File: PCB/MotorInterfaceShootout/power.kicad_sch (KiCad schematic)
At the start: 19 parts, among them U2 OPA4197, U3 LM7810, U4 LM79L05

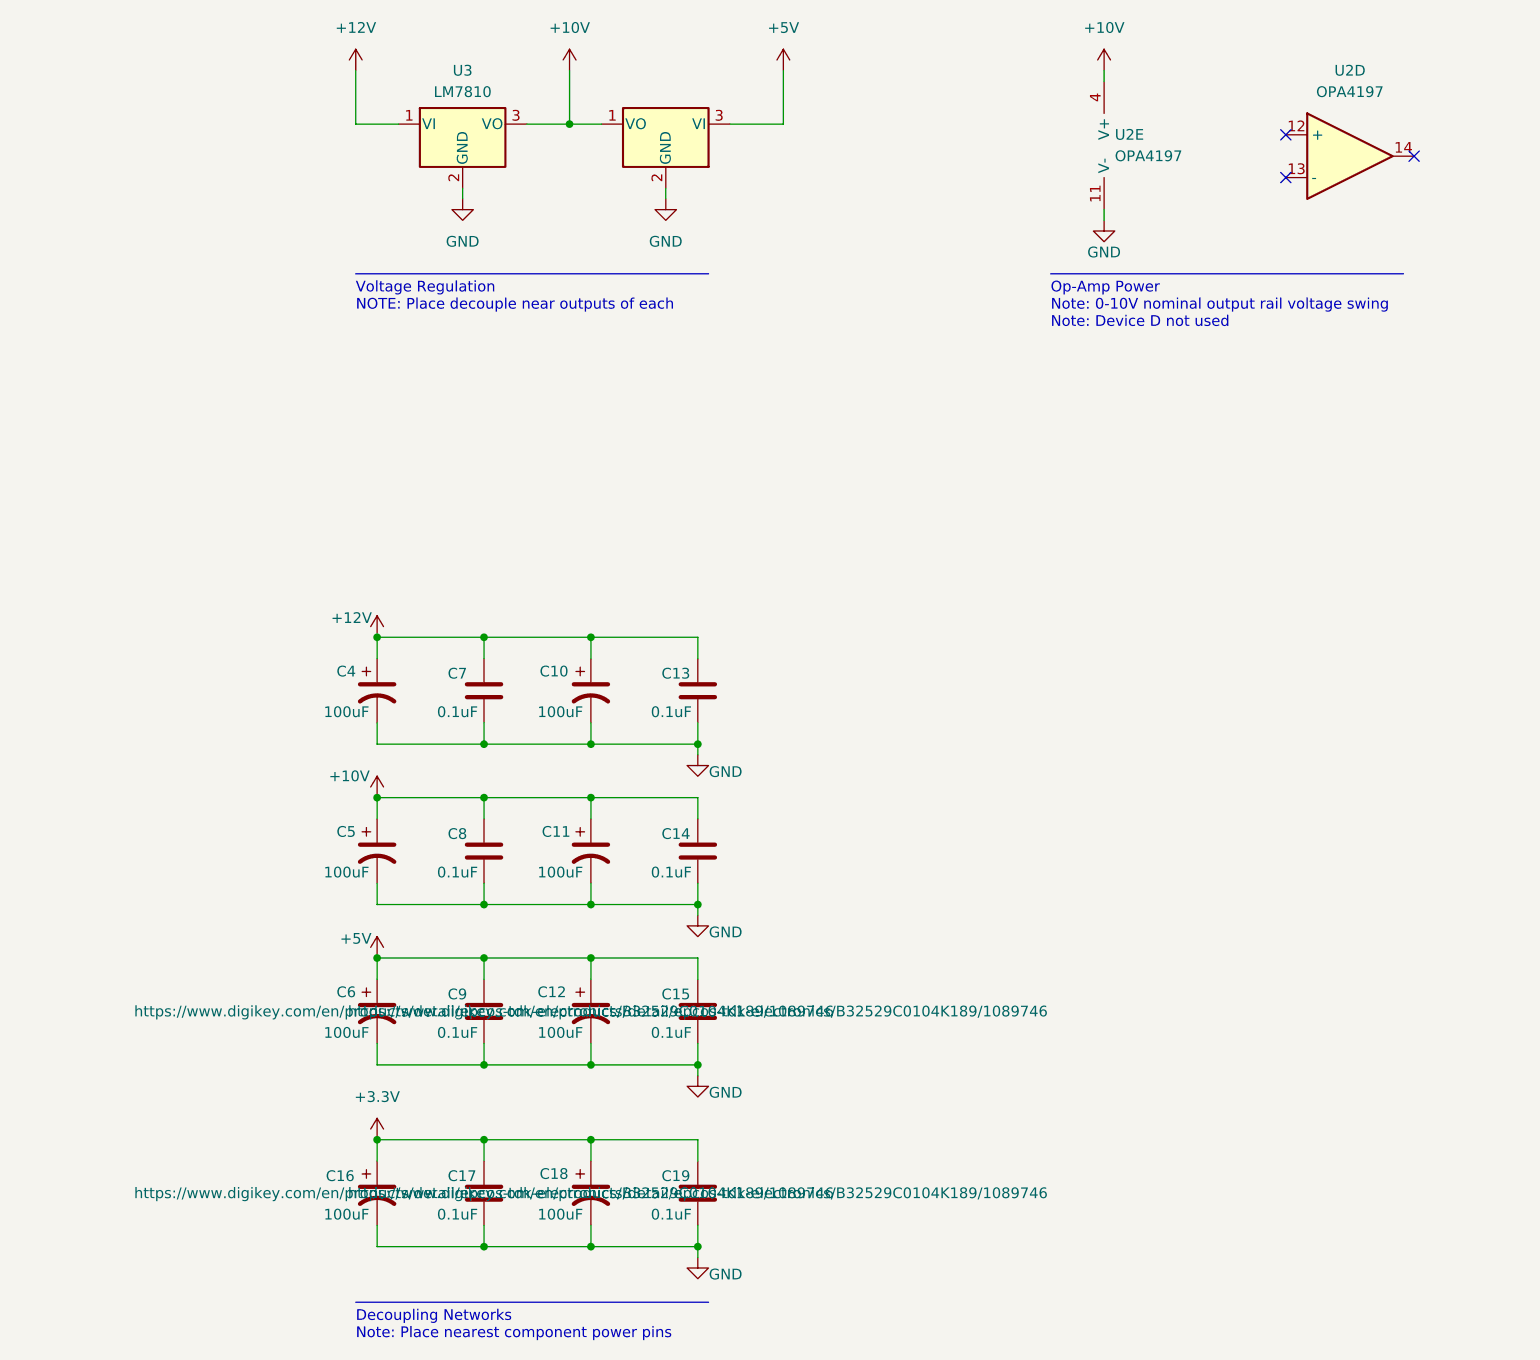
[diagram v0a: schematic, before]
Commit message: fix power
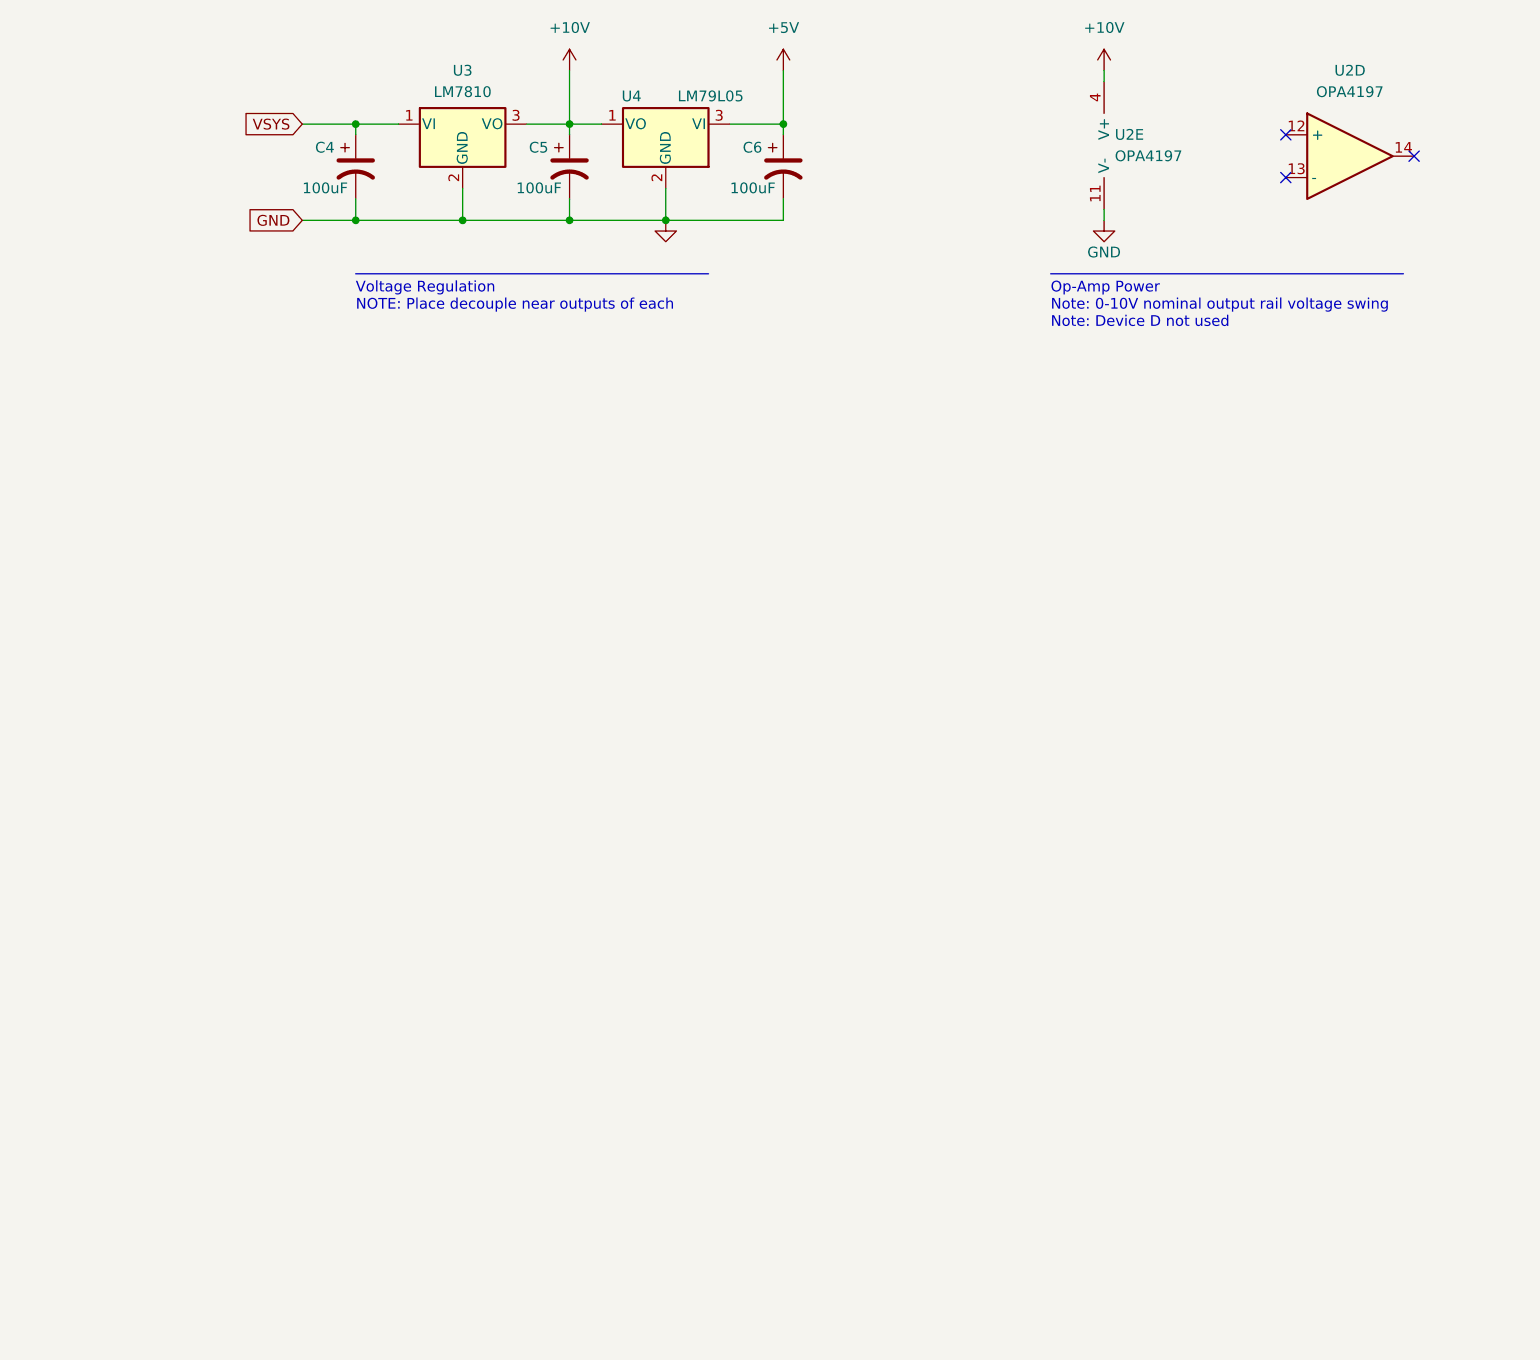
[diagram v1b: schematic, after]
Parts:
- removed C10, C11, C12, C16, C18: 100uF, TJR:C_Radial_D5.00mm_H12.5mm_P2.00mm, symbol TJR:C_Polarized_US
- removed C13, C14, C15, C17, C19, C7, C8, C9: 0.1uF, TJR:C_Rect_L7.3mm_W2.5_H6.5mm_P5.0mm, symbol Device:C
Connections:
- net +12V renamed VSYS
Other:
- note removed: "Decoupling Networks Note: Place nearest component power pins"
- moved on the sheet: C4
